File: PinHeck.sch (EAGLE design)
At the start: 343 parts, among them IC1 FT232RL-REEL, IC2 PIC32MX795F512L-80I/PT, IC3 CD74HCT244E, IC4 CD74HCT244E, IC5 ULN2803A, J1 500075-1517, J11 No Load, J2 500075-1517, J3 N/A, J6 161-3507-E, P1 TC33X-2-103E, SW1 101-0134-EV, SW2 101-0134-EV, SW3 101-0134-EV, SW4 0S102011MS2QS1, U1 P8X32A-Q44, U10 74HCT2G04GV,125, U11 74HC165D,652, U12 74HC165D,652, U14 MC74HC08ADG, U15 MC74HC08ADG, U16 MC74HC08ADG, U17 MC74HC08ADG, U18 MC74HC08ADG, U19 MC74HC08ADG, U2 FT230XS-R, U20 TIP107, U21 TIP107, U22 TIP107, U23 TIP107, U24 TIP107, U25 TIP107, U26 TIP107, U27 TIP107, U28 TIP102, U29 TIP102, U3 74HC595D-Q100, U30 TIP102, U31 TIP102, U32 TIP102, U33 TIP102, U34 TIP102, U35 TIP102, U36 WS2801, U37 TIP102, U38 WS2801, U39 LM2937IMP-3.3/NOPB, U4 24LC1025-I/P, U40 TIP102, U41 TIP102, U42 TIP102, U43 TIP102, U44 TIP102, U45 TIP102, U46 TIP102, U47 TIP102, U48 TIP102, U49 TIP102, U5 74HC595D-Q100, U50 TIP102, U51 TIP102, U52 CD74HC123M96, U6 TIP102, U7 TIP102, U8 TIP102, U9 TIP102, X1 FQ7050B-8.000, X2 ECS-65-20-4X

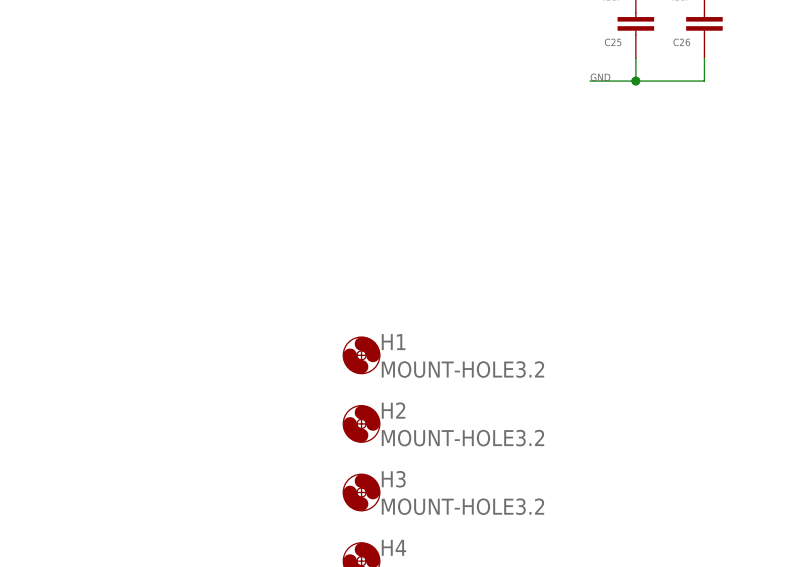
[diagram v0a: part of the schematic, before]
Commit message: Added MF Logo
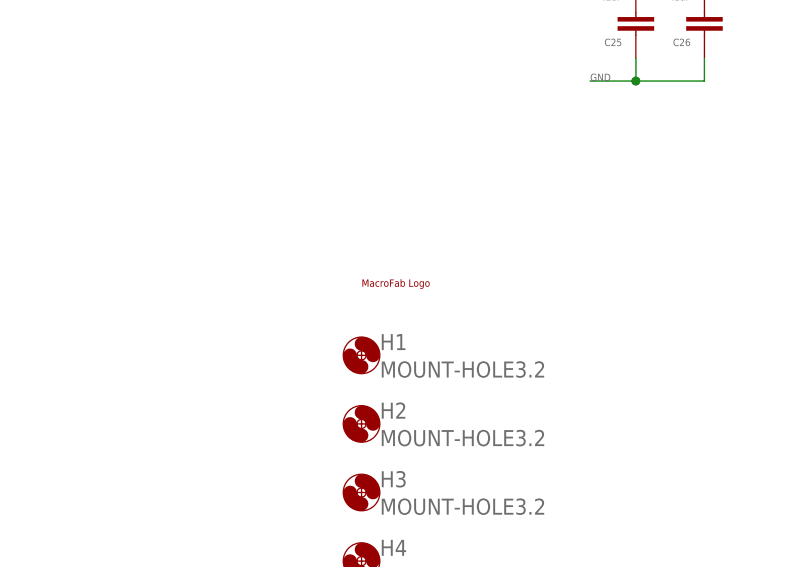
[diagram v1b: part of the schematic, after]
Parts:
- added U$2: MF_LOGOLOGO_TEXT, PP_Aesthetics:MF_LOGOLOGO_TEXT
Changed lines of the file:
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@@
 <part name="R140" library="PP_Passives" deviceset="RESISTOR" device="0805" value="4.7K"/>
 <part name="R141" library="PP_Passives" deviceset="RESISTOR" device="0805" value="4.7K"/>
+<part name="U$2" library="PP_Aesthetics" deviceset="MF_LOGO" device="LOGO_TEXT"/>
 </parts>
 <sheets>
@@
 <instance part="R140" gate="G$1" x="248.92" y="17.78" rot="R90"/>
 <instance part="R141" gate="G$1" x="274.32" y="17.78" rot="R90"/>
+<instance part="U$2" gate="G$1" x="307.34" y="-63.5"/>
 </instances>
 <busses>
